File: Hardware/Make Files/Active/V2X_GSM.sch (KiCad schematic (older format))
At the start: 46 parts, among them P1 SIM_SKT, P14 CUR_SEN, P2 SMA, P26 CONN_02X10, P3 SMA, Q12 IRF9335, U13 XRP6124, U3 MMQA5V6T3G, U4 SIM5320

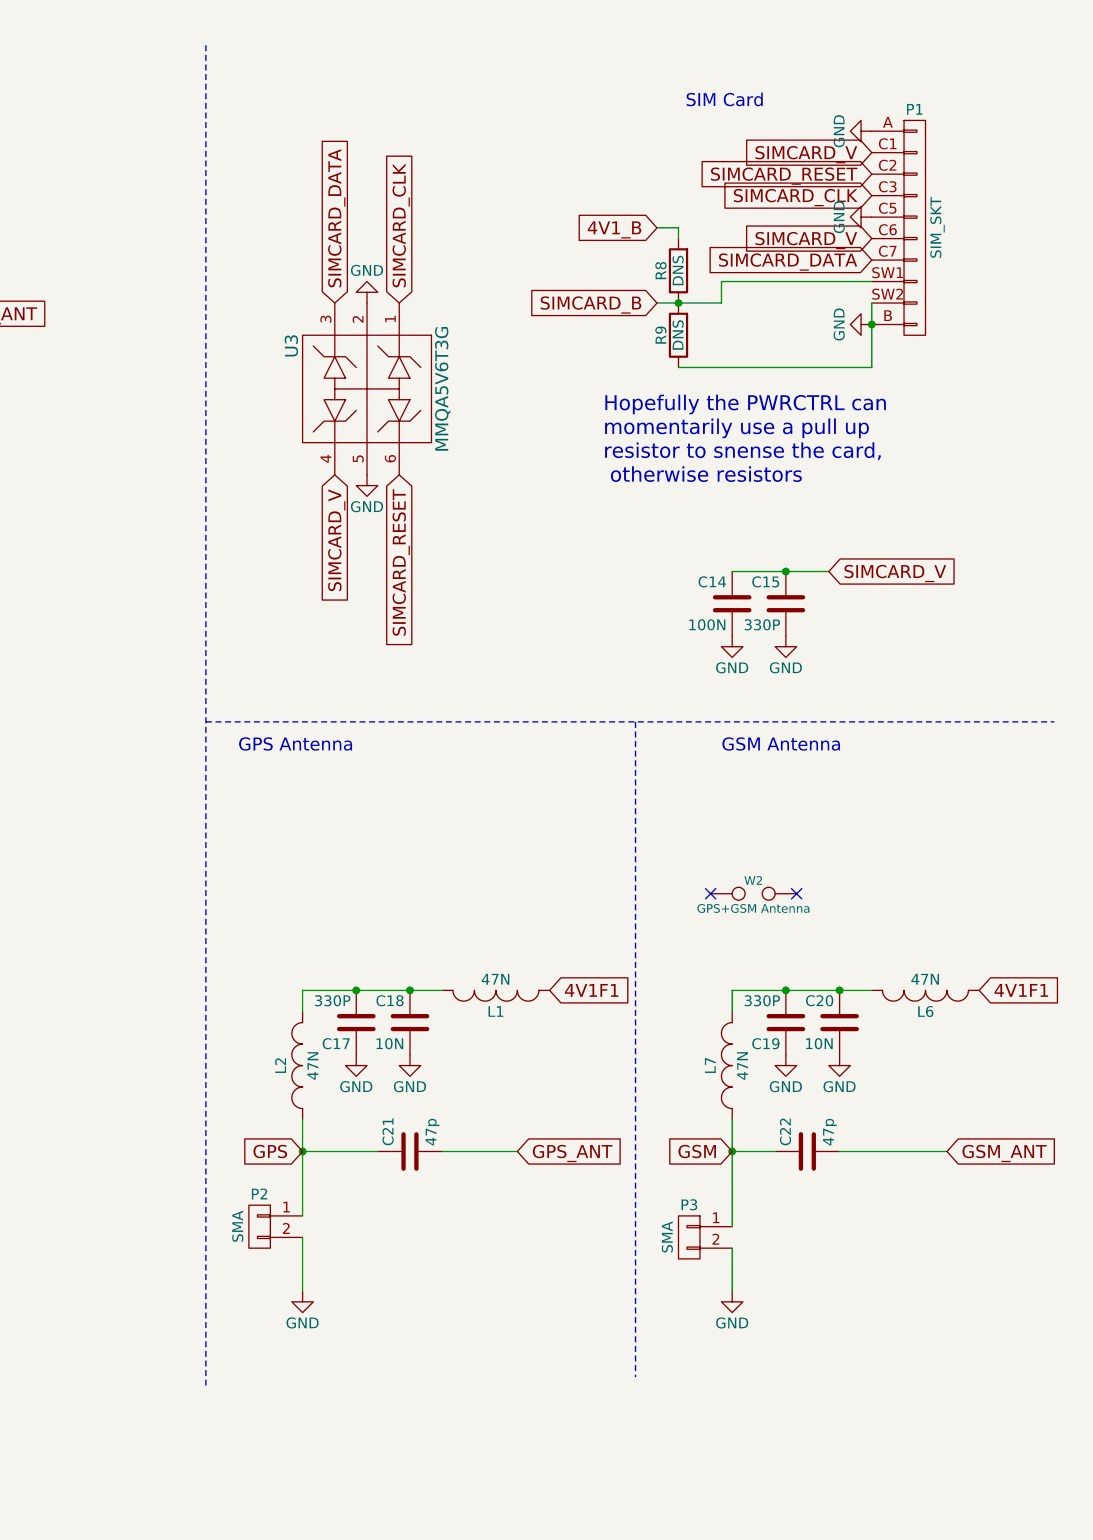
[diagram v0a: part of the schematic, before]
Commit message: V1.2 Ordered
This is a capture of the project folder at the time f ordering the V1.2
kit.
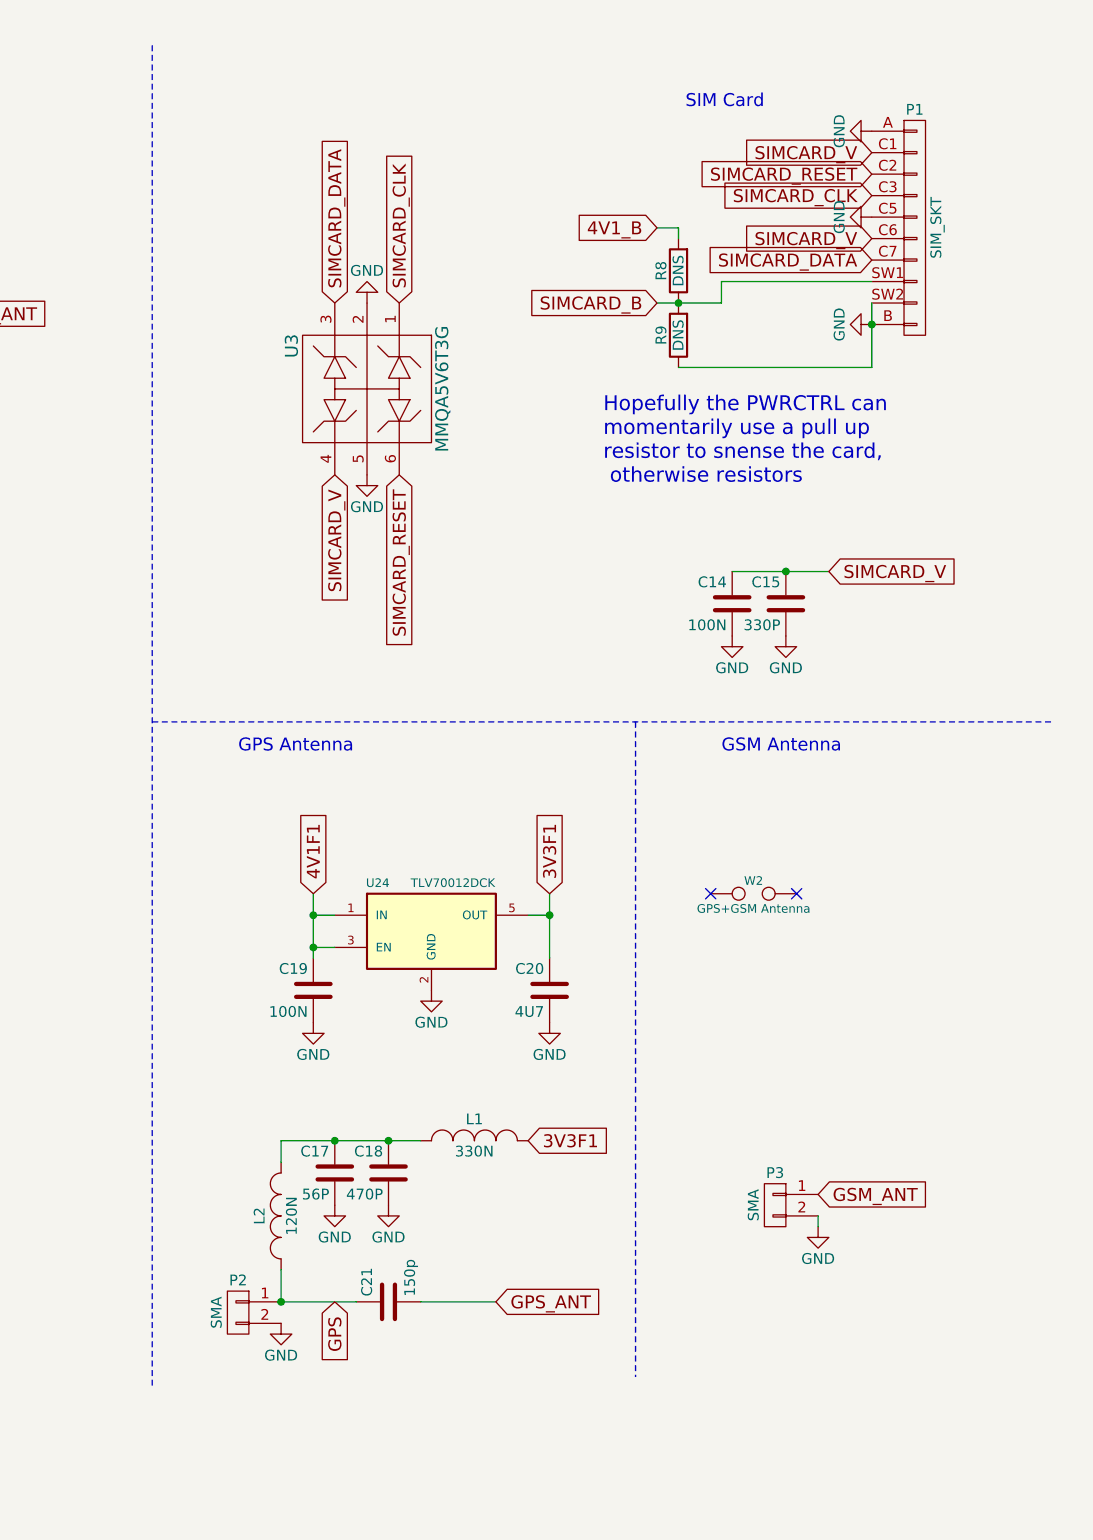
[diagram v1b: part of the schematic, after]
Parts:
- removed C22: 47p, Custom Parts:C_0603_SM, symbol C
- removed L6, L7: 47N, Custom Parts:C_0603_SM, symbol INDUCTOR_SMALL
- added U24: TLV70012DCK, symbol TLV70012DCK
- C17: value 330P -> 56P; Mouse PN 77-VJ0603D331KXAAJ -> 581-08052U560G
- C18: value 10N -> 470P; Mouse PN 77-VJ0603Y103KXACBC -> 77-VJ0603D471KXXAJ
- C19: value 330P -> 100N; Mouse PN 77-VJ0603D331KXAAJ -> 810-C1608X7R1E104K
- C20: value 10N -> 4U7; footprint Custom Parts:C_0603_SM -> Custom Parts:C_0805_SM; Mouse PN 77-VJ0603Y103KXACBC -> 581-12063C475KAT2A
- C21: value 47p -> 150p; Mouse PN 80-CBR06C470J5G -> 77-VJ0805Q151JXAAC
- L1: value 47N -> 330N
- L2: value 47N -> 120N; Mouse PN 81-LQG18HN47NJ00D -> 81-LQW18CNR12J00D
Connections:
- net GSM is gone; now on net GSM_ANT: P3.1 (P1)
- net 4V1F1: now also C19.1, U24.1 (IN), U24.3 (EN); no longer L1.1
- net GND: now also C17.2, C19.2, U24.2 (GND); no longer C17.1, C19.1
- net at C18.1, L1.2, L2.2: now also C17.1; no longer C17.2
- net 3V3F1: now reaches C20.1
- net 3V3F1: now also L1.1, U24.5 (OUT); no longer C19.2
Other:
- moved on the sheet: C17, C18, C21, L1, L2, P2, P3
